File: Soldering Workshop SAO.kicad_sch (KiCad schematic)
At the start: 18 parts, among them J1 Conn_02x03_Odd_Even, M1 220, SW1 SW_SPDT, T1 220, U1 LMC555xM

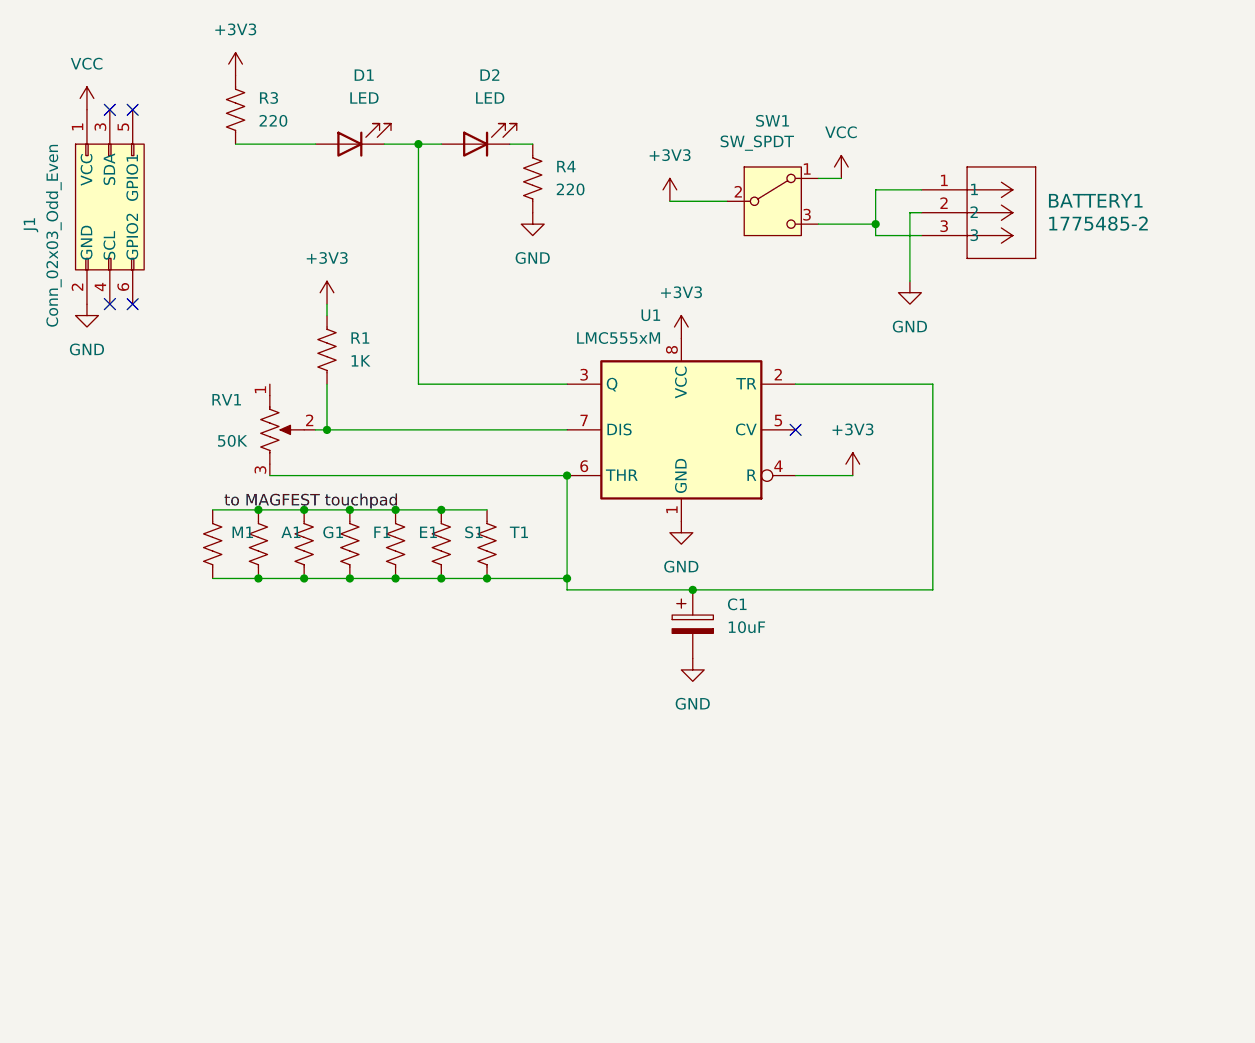
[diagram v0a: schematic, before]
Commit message: cleanup data, readme
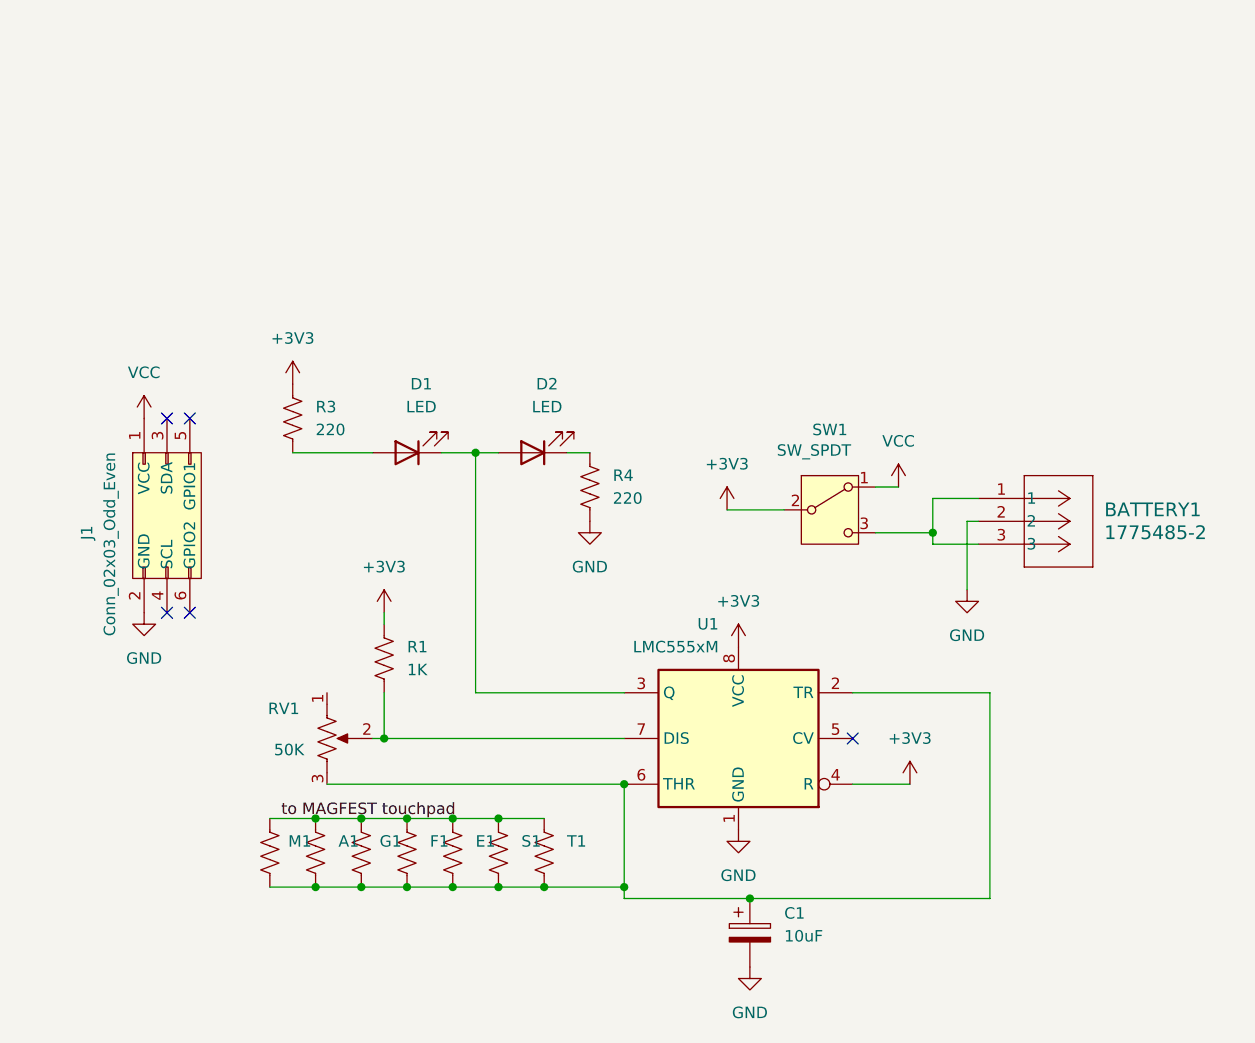
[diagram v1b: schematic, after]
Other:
- company: (none) -> MAGFEST INC
- title: (none) -> 2025 MAGFEST SOLDERING WORKSHOP
- moved on the sheet: A1, BATTERY1, C1, D1, D2, E1, F1, G1, J1, M1, R1, R3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
